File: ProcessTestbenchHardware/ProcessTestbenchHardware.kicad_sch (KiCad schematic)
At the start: 52 parts, among them J1 Screw_Terminal_01x02, J10 Screw_Terminal_01x02, J2 ModuloRS485, J8 DB15, J9 Screw_Terminal_01x02, Q1 IRLZ44N, Q2 IRLZ44N, Q3 IRLZ44N, Q4 IRF540N, Q5 IRLZ44N, Q6 IRLZ44N, U2 StepDownConverter, U3 ICL7660, U4 AD620, U5 AD620, U6 LM358

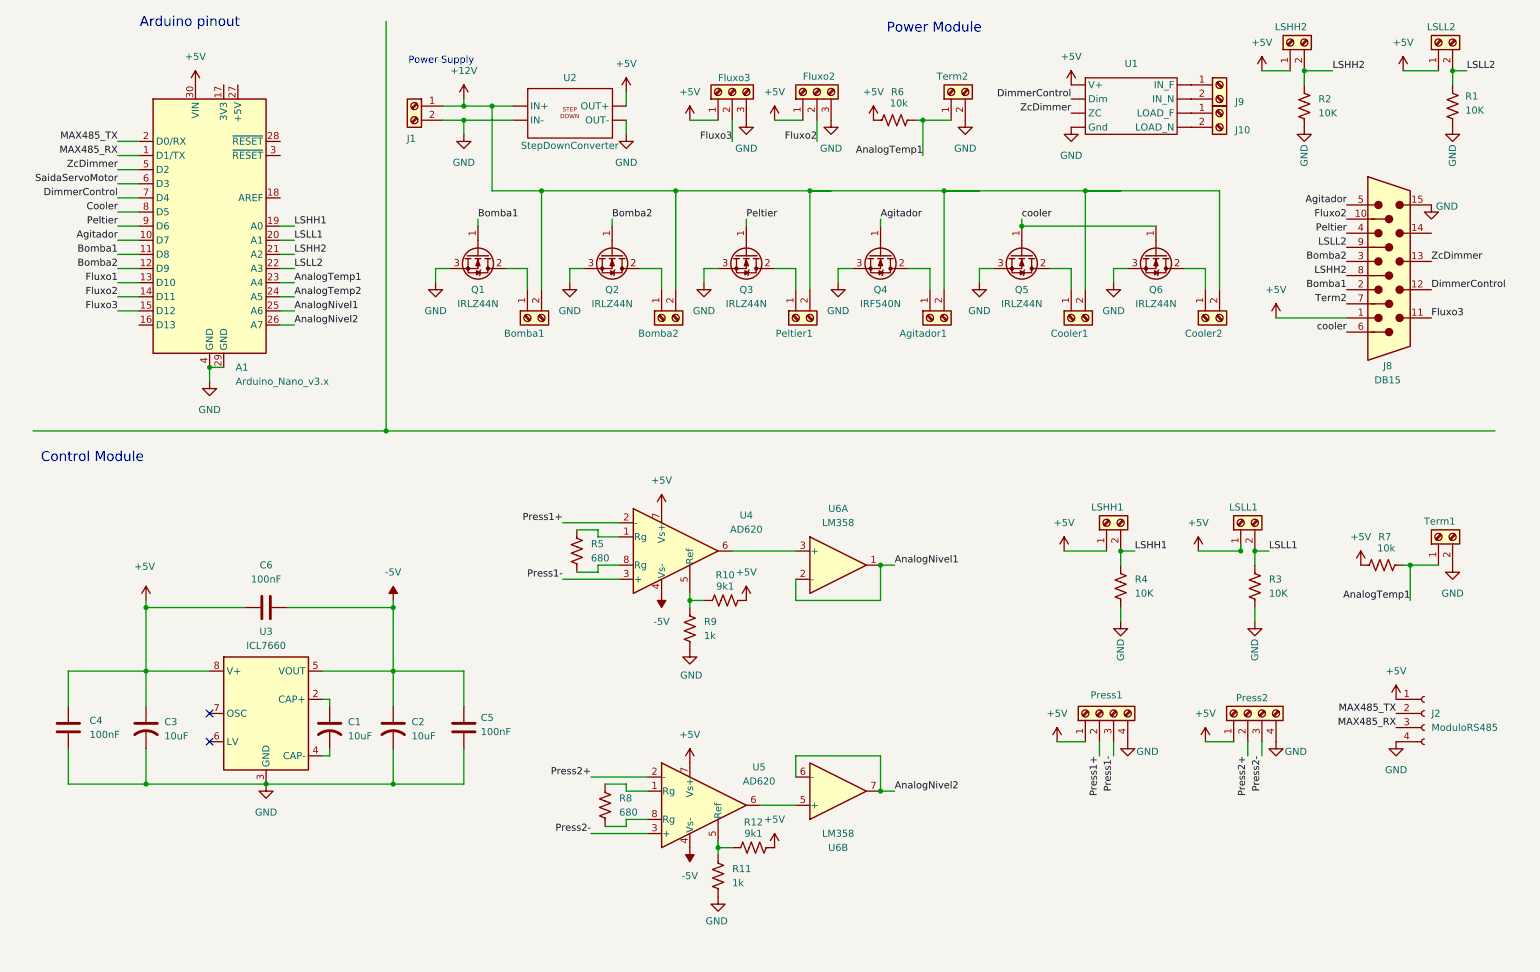
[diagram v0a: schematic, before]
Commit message: ScrewTerminalsForDimmer
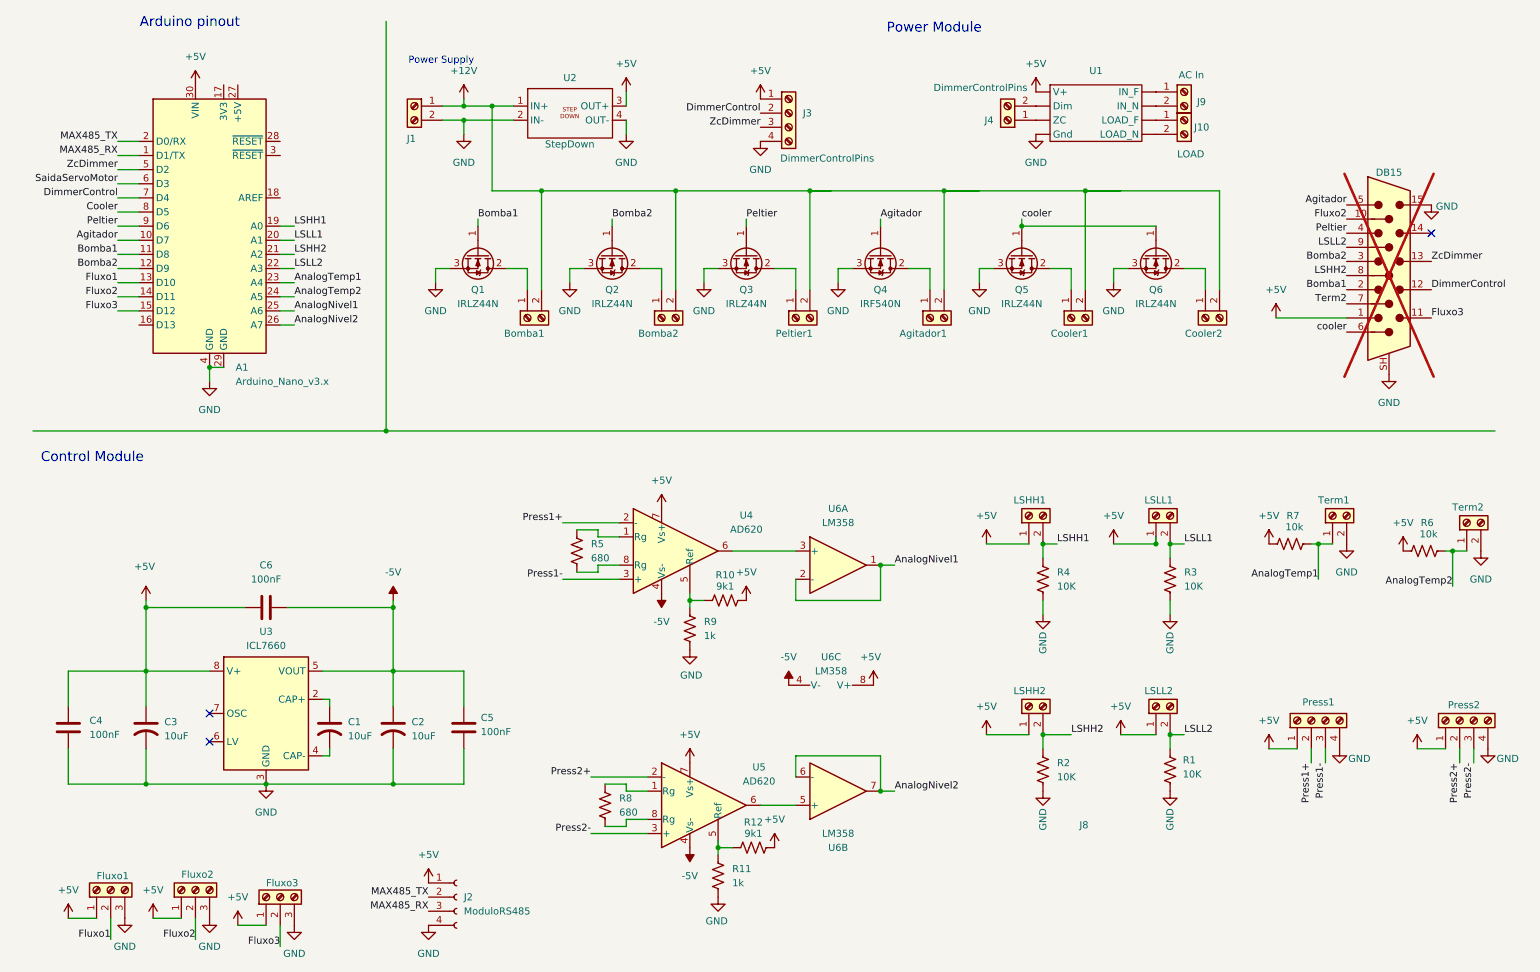
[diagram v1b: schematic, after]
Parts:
- added Fluxo1: Screw_Terminal_01x03, TerminalBlock:TerminalBlock_MaiXu_MX126-5.0-03P_1x03_P5.00mm, symbol Connector:Screw_Terminal_01x03
- added J3: DimmerControlPins, TerminalBlock:TerminalBlock_MaiXu_MX126-5.0-04P_1x04_P5.00mm, symbol Connector:Screw_Terminal_01x04
- added J4: DimmerControlPins, symbol Connector:Screw_Terminal_01x02
- added unit 3 of U6
- Agitador1: value Screw_Terminal_01x02 -> Agitador1
- Bomba1: value Screw_Terminal_01x02 -> Bomba1
- Bomba2: value Screw_Terminal_01x02 -> Bomba2
- Cooler1: value Screw_Terminal_01x02 -> Cooler1
- Cooler2: value Screw_Terminal_01x02 -> Cooler2
- J10: value Screw_Terminal_01x02 -> LOAD; now left out of the parts list
- J8: symbol Connector:DE15_Pins_HighDensity -> Connector:DE15_Pins_HighDensity_MountingHoles; now not fitted; now left out of the parts list
- J9: value Screw_Terminal_01x02 -> AC In; now left out of the parts list
- LSHH1: value Screw_Terminal_01x02 -> LSHH1
- LSHH2: value Screw_Terminal_01x02 -> LSHH2
- LSLL1: value Screw_Terminal_01x02 -> LSLL1
- LSLL2: value Screw_Terminal_01x02 -> LSLL2
- Peltier1: value Screw_Terminal_01x02 -> Peltier1
- Press1, Press2: value Screw_Terminal_01x04 -> Press1
- Term1: value Screw_Terminal_01x02 -> Term1
- Term2: value Screw_Terminal_01x02 -> Term2
- U2: value StepDownConverter -> StepDown; footprint AddOnsLibrary:StepDownFootprint -> AddOnsLibrary:SRT_MPT1584EN_Module
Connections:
- net +12V: now also U2.1 (IN+); no longer U2. (OUT-)
- net +5V: now also U2.3 (OUT+), Fluxo1.1 (Pin_1), J3.1 (Pin_1), U6.8 (V+); no longer U2. (OUT-)
- net -5V: now also U6.4 (V-)
- net AnalogTemp1: no longer R6.2, Term2.1 (Pin_1)
- net AnalogTemp2: now also R6.2, Term2.1 (Pin_1)
- net DimmerControl: now also J3.2 (Pin_2); no longer U1. (LOAD_N)
- net Fluxo1: now also Fluxo1.2 (Pin_2)
- net GND: now also J8.SH, U2.2 (IN-), U2.4 (OUT-), Fluxo1.3 (Pin_3), J3.4 (Pin_4); no longer U2. (OUT-)
- net ZcDimmer: now also J3.3 (Pin_3); no longer U1. (LOAD_N)
- new net: J4.1 (Pin_1), U1. (LOAD_N)
- new net: J4.2 (Pin_2), U1. (LOAD_N)
- no-connect marks 2 -> 3
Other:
- moved on the sheet: Fluxo2, Fluxo3, J10, J2, J9, LSHH1, LSHH2, LSLL1, LSLL2, Press1, Press2, R1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
